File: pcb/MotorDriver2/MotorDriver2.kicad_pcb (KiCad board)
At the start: 4 copper layers, 77 x 82 mm, 125 parts, among them IC1 STM32C092RCT6, IC2 CP2102N-A02-GQFN20R, J1 USB4110-GF-A, J2 Conn_01x02, J3 Conn_01x02, J4 Conn_01x02, J5 Conn_01x02, J6 Conn_01x04, Q1 IRLZ44NSTRLPBF, Q2 IRLZ44NSTRLPBF, Q3 IRLZ44NSTRLPBF, Q4 IRLZ44NSTRLPBF, Q5 IRLZ44NSTRLPBF, Q6 IRLZ44NSTRLPBF, Q7 IRLZ44NSTRLPBF, Q8 IRLZ44NSTRLPBF, SW1 K2-6639SP-C4SC-04, SW2 K2-6639SP-C4SC-04, SW3 K2-6639SP-C4SC-04, U1 NCP361SNT1G, U2 MAX40200AUK, U3 XIAO-ESP32-C5-DIP, U6 LM324DR, U7 USBLC6-2SC6, Y1 48 MHz, Y2 32.768 kHz

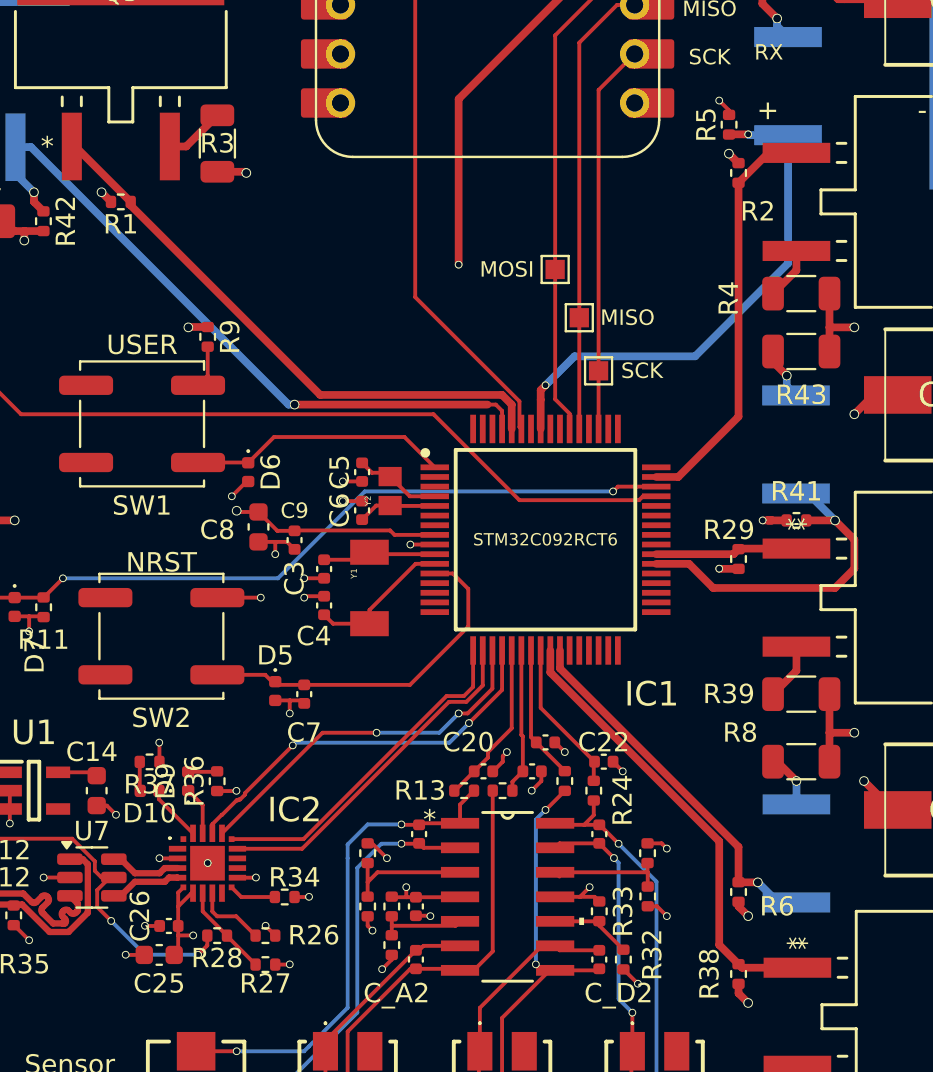
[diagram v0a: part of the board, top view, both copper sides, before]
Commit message: Added step files
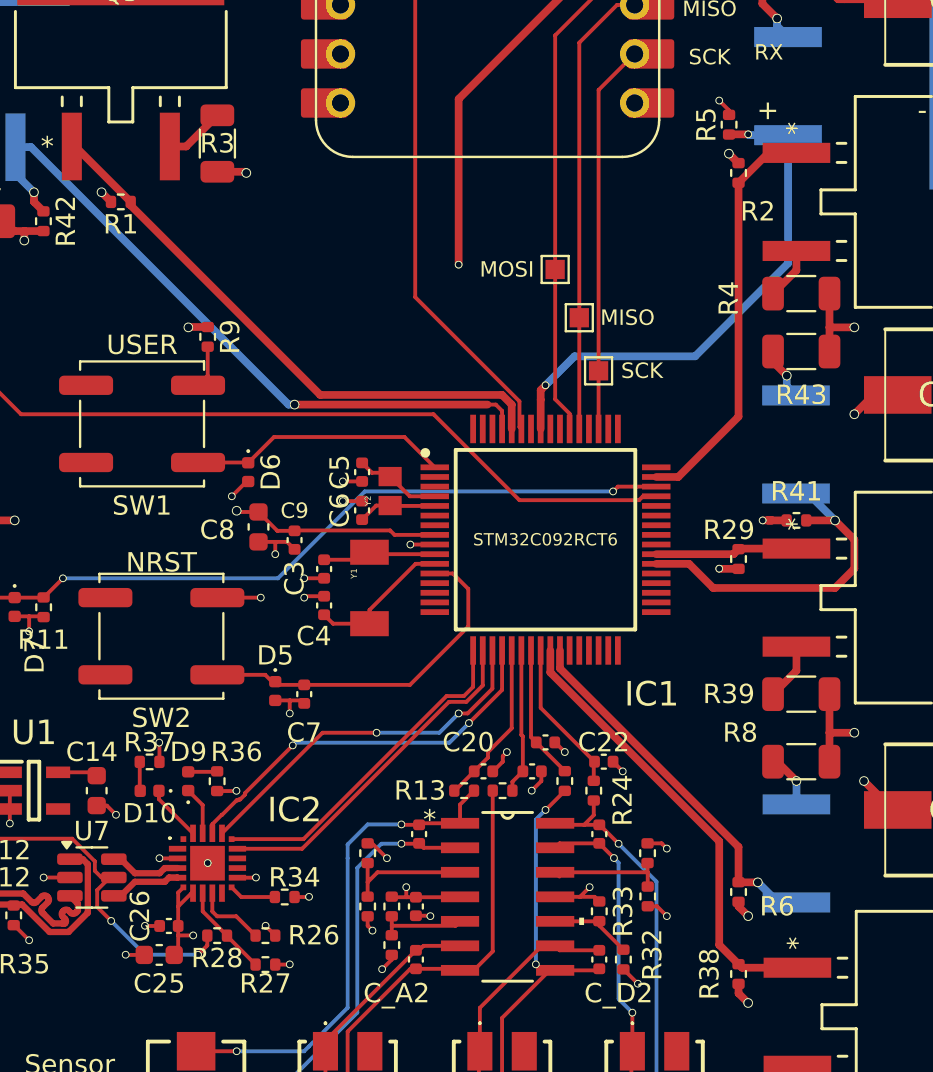
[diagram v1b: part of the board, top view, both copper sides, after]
